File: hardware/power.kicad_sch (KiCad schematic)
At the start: 35 parts

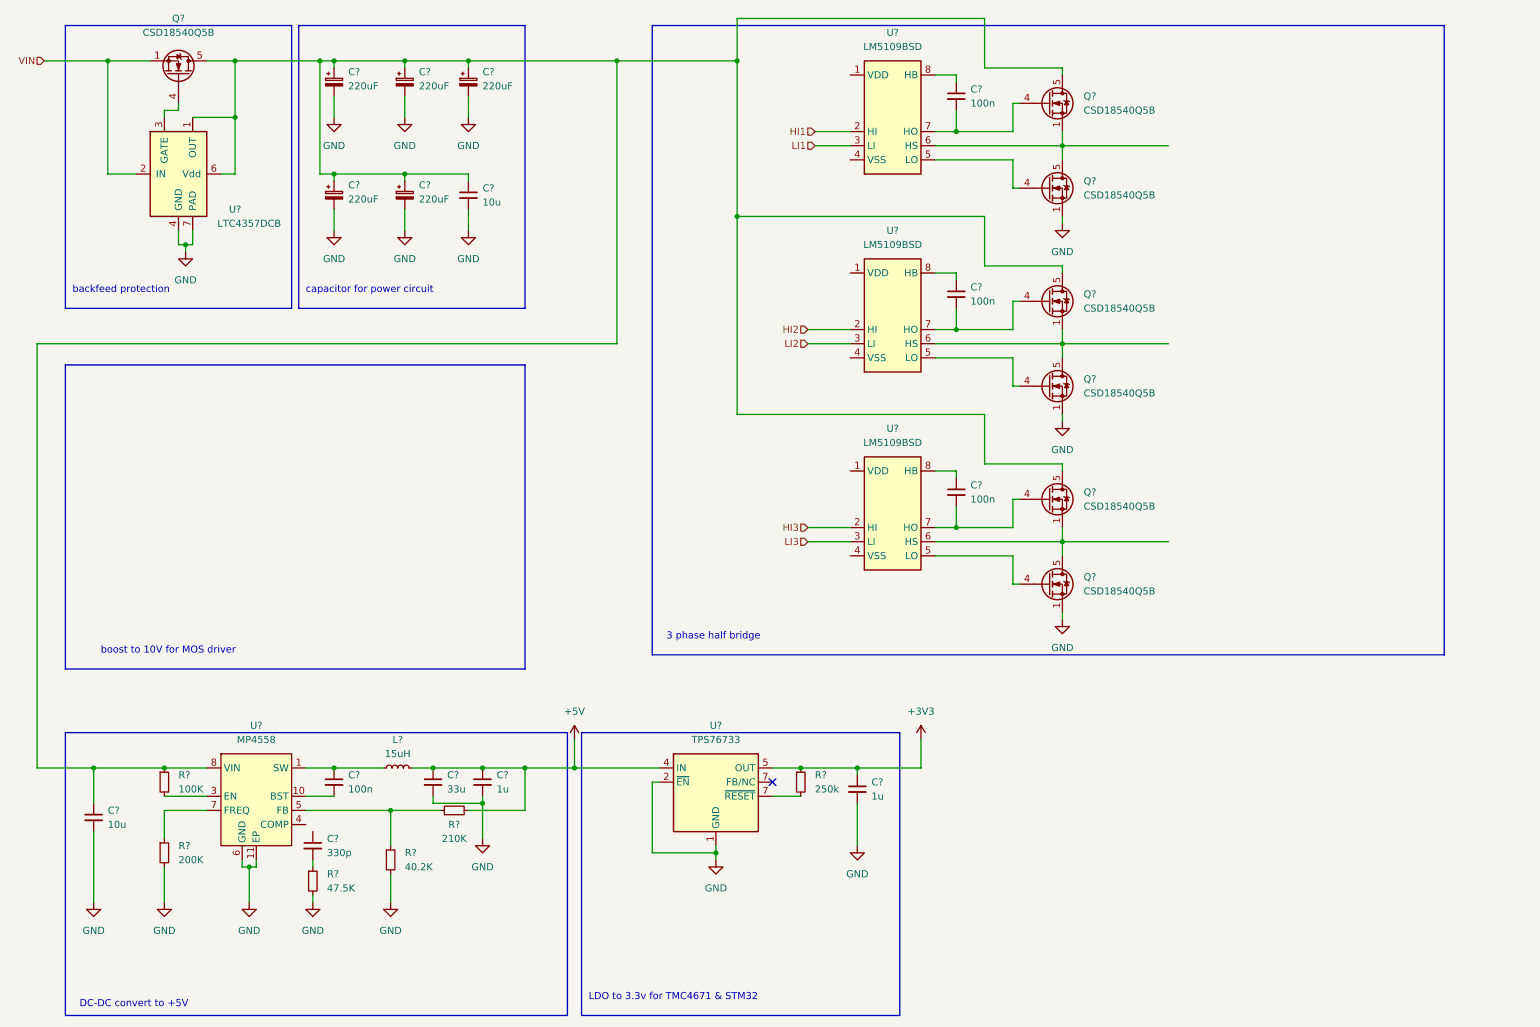
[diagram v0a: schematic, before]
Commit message: finish power tree
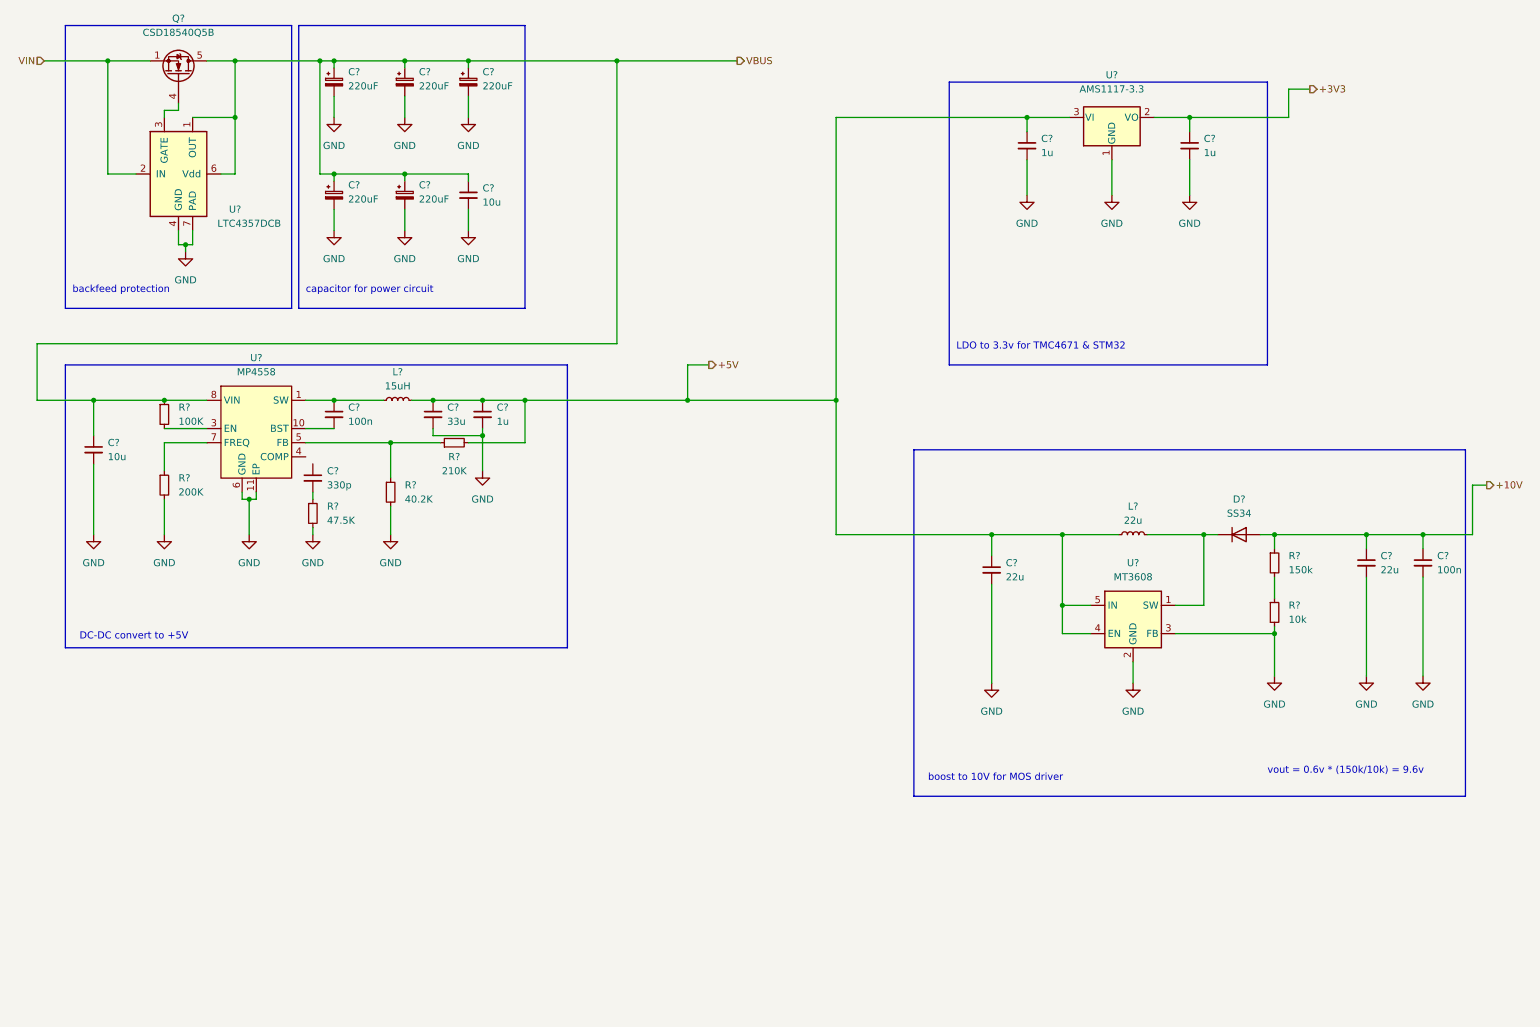
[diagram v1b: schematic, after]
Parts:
- removed C? (x3): 100n, symbol Device:C_Small
- removed C?: 1u, symbol Device:C_Small
- removed Q? (x6): CSD18540Q5B, Package_TO_SOT_SMD:TDSON-8-1, symbol Transistor_FET:CSD18540Q5B
- removed R?: 250k, symbol Device:R_Small
- removed U? (x3): LM5109BSD, Package_SON:WSON-8-1EP_4x4mm_P0.8mm_EP2.6x3mm, symbol Driver_FET:LM5109BSD
- removed U?: TPS76733, Package_SO:SOIC-8_3.9x4.9mm_P1.27mm, symbol Regulator_Linear:TPS76733
- added C? (x2): 1u, symbol Device:C_Small
- added C? (x2): 22u, symbol Device:C_Small
- added C?: 100n, symbol Device:C_Small
- added D?: SS34, Diode_THT:D_DO-35_SOD27_P7.62mm_Horizontal, symbol Diode:1N4148
- added L?: 22u, symbol Device:L_Small
- added R?: 150k, symbol Device:R_Small
- added R?: 10k, symbol Device:R_Small
- added U?: MT3608, Package_TO_SOT_SMD:SOT-23-6, symbol Regulator_Switching:MT3608
- added U?: AMS1117-3.3, Package_TO_SOT_SMD:SOT-223-3_TabPin2, symbol Regulator_Linear:AMS1117-3.3
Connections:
- net +3V3: now also C?.1, U?.2 (VO)
- net +5V: now also C?.1, C?.1, L?.1, U?.3 (VI), U?.4 (EN), U?.5 (IN)
- net GND: now also C?.2, C?.2, C?.2, C?.2, C?.2, R?.2, U?.1 (GND), U?.2 (GND), U?.3 (FB)
- new net: D?.1 (K), L?.2, U?.1 (SW)
- new net: R?.1, R?.2
- new net +10V: C?.1, C?.1, D?.2 (A), R?.1
- no-connect marks 1 -> 0
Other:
- note added: "vout = 0.6v * (150k/10k) = 9.6v"
- note removed: "3 phase half bridge"
- moved on the sheet: C?, L?, R?, U?
